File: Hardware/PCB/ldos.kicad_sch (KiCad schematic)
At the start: 8 parts, among them U10 AZ1117-5.0, U4 AP7361C-33E

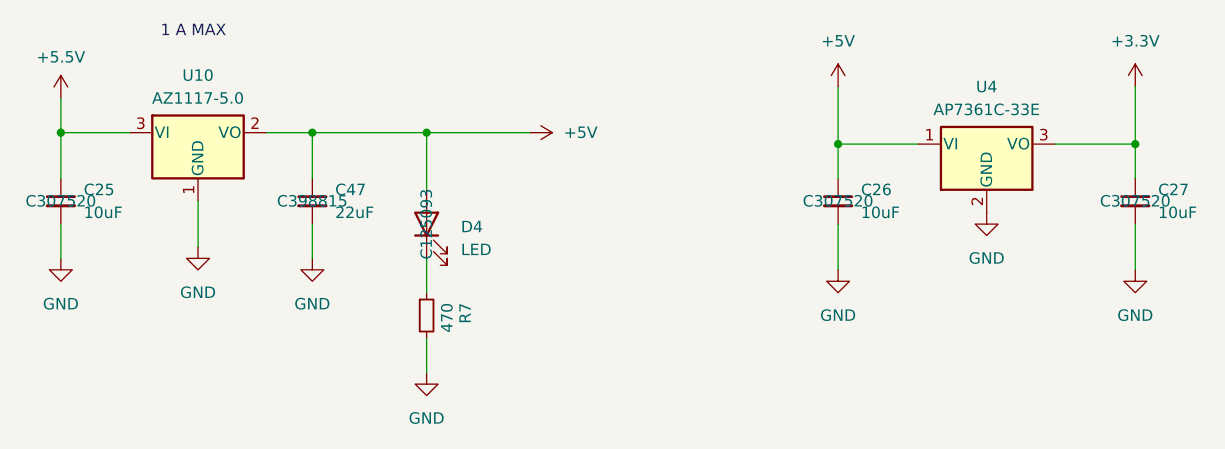
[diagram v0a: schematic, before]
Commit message: done with this, placed order
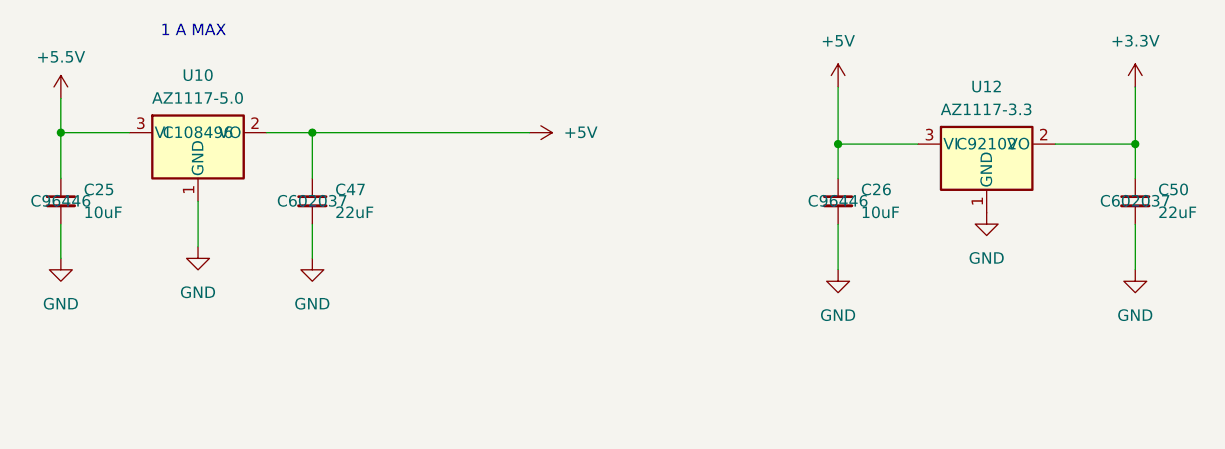
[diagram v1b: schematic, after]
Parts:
- removed C27: 10uF, Capacitor_SMD:C_0805_2012Metric_Pad1.18x1.45mm_HandSolder, symbol Device:C_Small
- removed D4: LED, LED_SMD:LED_0603_1608Metric_Pad1.05x0.95mm_HandSolder, symbol Device:LED
- removed R7: 470, Resistor_SMD:R_0603_1608Metric_Pad0.98x0.95mm_HandSolder, symbol Device:R_Small
- removed U4: AP7361C-33E, Package_TO_SOT_SMD:SOT-223-3_TabPin2, symbol Regulator_Linear:AP7361C-33E
- added C50: 22uF, Capacitor_SMD:C_0805_2012Metric_Pad1.18x1.45mm_HandSolder, symbol Device:C_Small
- added U12: AZ1117-3.3, Package_TO_SOT_SMD:SOT-223-3_TabPin2, symbol Regulator_Linear:AZ1117-3.3
- C25, C26: footprint Capacitor_SMD:C_0805_2012Metric_Pad1.18x1.45mm_HandSolder -> Capacitor_SMD:C_0603_1608Metric_Pad1.08x0.95mm_HandSolder; LCSC C307520 -> C96446; MPN CL21A106KOQNNNG -> CL10A106MA8NRNC
- C47: LCSC C398815 -> C602037; MPN CL21A226MOCLRNC -> CL21A226MAYNNNE
- U10: LCSC (none) -> C108496
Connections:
- net +3.3V: now also C50.1, U12.2 (VO)
- net +5V: now also U12.3 (VI)
- net GND: now also C50.2, U12.1 (GND)
